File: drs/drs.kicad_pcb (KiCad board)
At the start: 2 copper layers, 68.5 x 53.5 mm, 26 parts, among them J1 CAN, J2 POWER, J3 BUTTON, J4 SERVO, U1 SN65HVD230, U2 TXU0202

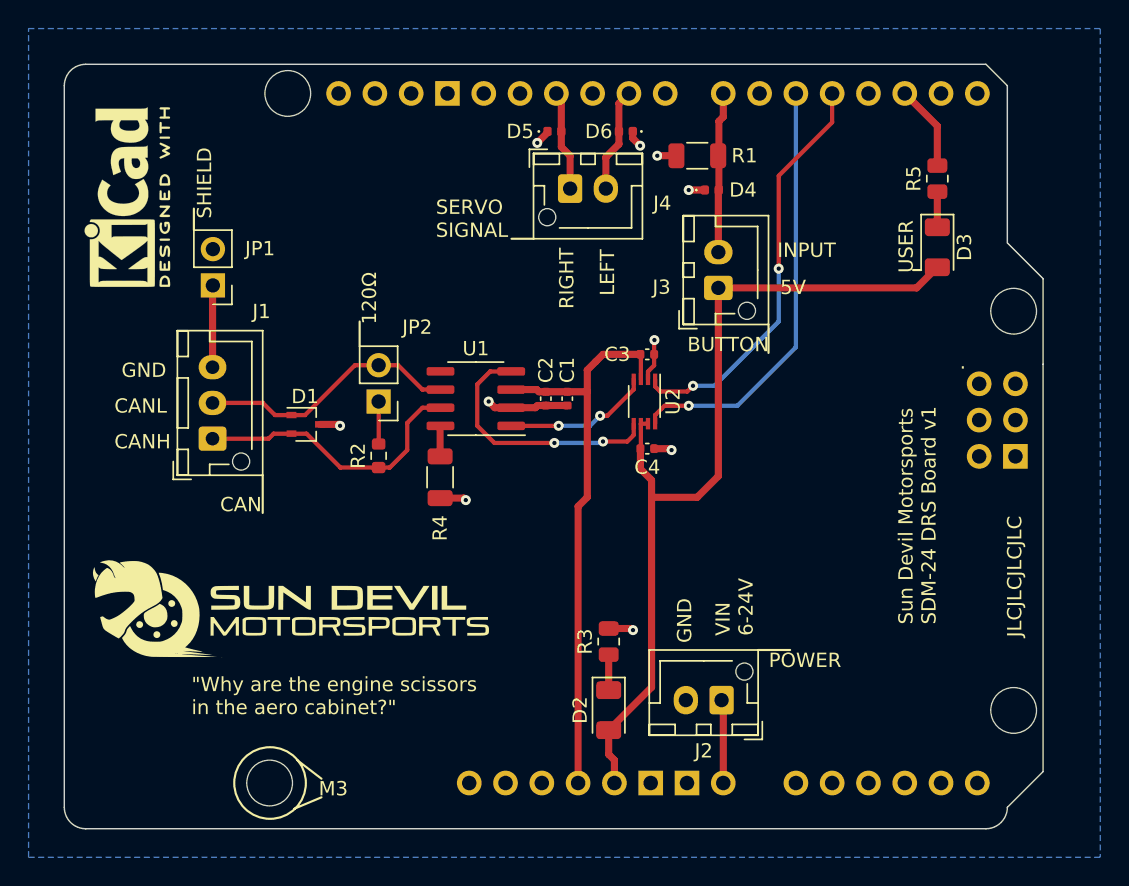
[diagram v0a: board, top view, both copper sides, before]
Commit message: fahb files
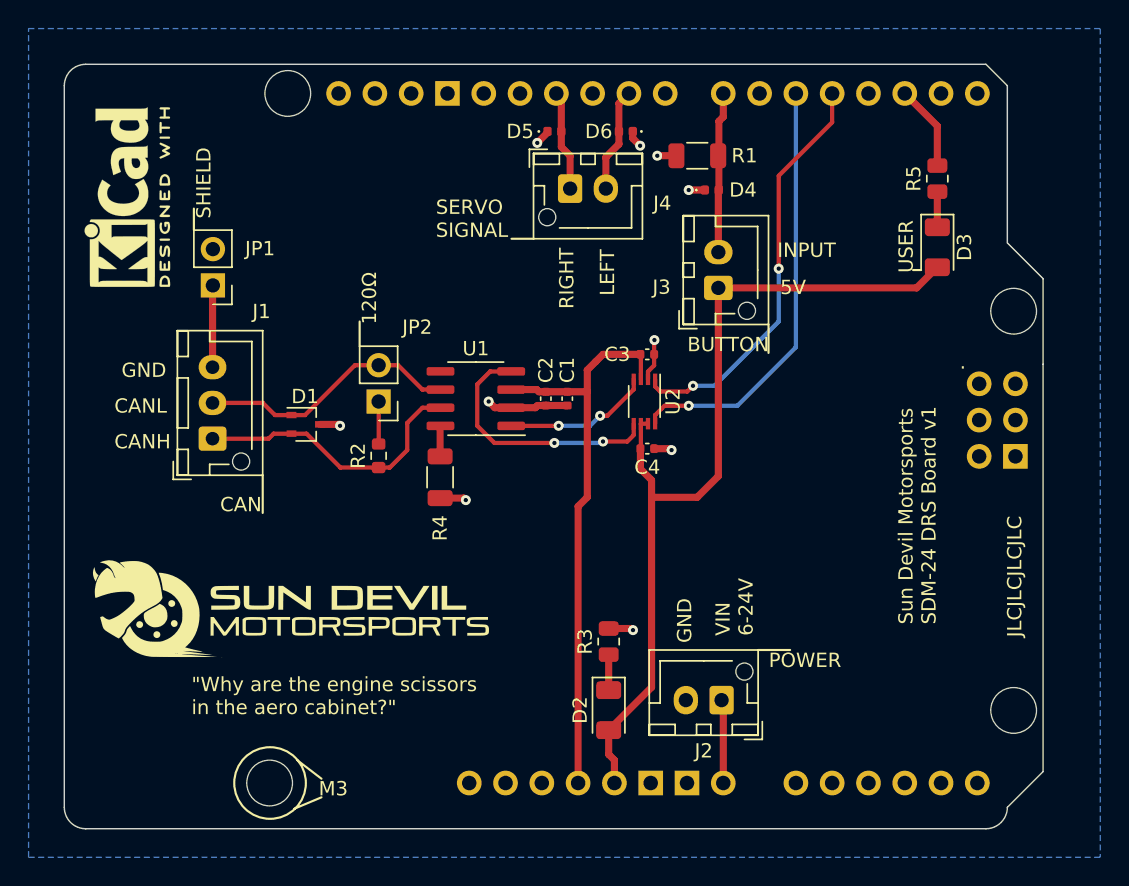
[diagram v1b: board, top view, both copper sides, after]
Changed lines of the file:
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@@
       (plot_on_all_layers_selection 0x0000000_00000000)
       (disableapertmacros false)
-      (usegerberextensions false)
-      (usegerberattributes true)
-      (usegerberadvancedattributes true)
-      (creategerberjobfile true)
+      (usegerberextensions true)
+      (usegerberattributes false)
+      (usegerberadvancedattributes false)
+      (creategerberjobfile false)
       (dashed_line_dash_ratio 12.000000)
       (dashed_line_gap_ratio 3.000000)
@@
       (psa4output false)
       (plotreference true)
-      (plotvalue true)
+      (plotvalue false)
       (plotinvisibletext false)
       (sketchpadsonfab false)
-      (subtractmaskfromsilk false)
+      (subtractmaskfromsilk true)
       (outputformat 1)
       (mirror false)
-      (drillshape 1)
+      (drillshape 0)
       (scaleselection 1)
-      (outputdirectory "")
+      (outputdirectory "fab/")
     )
   )
@@
       (stroke (width 0.1) (type solid)) (layer "F.Fab"))
     (pad "" np_thru_hole circle (at -1.6 2 90) (size 1.2 1.2) (drill 1.2) (layers "*.Cu" "*.Mask"))
-    (pad "1" thru_hole roundrect (at 0 0 90) (size 1.7 2) (drill 1) (layers "*.Cu" "*.Mask") (roundrect_rratio 0.147059)
+    (pad "1" thru_hole roundrect (at 0 0 90) (size 1.7 2) (drill 1) (layers "*.Cu" "*.Mask") (roundrect_rratio 0.1470588235)
       (net 40 "+5V") (pinfunction "Pin_1") (pintype "passive"))
     (pad "2" thru_hole oval (at 2.5 0 90) (size 1.7 2) (drill 1) (layers "*.Cu" "*.Mask")
@@
     (fp_line (start 1.6 0.8) (end -1.6 0.8)
       (stroke (width 0.1) (type solid)) (layer "F.Fab"))
-    (pad "1" smd roundrect (at -1.4625 0 180) (size 1.125 1.75) (layers "F.Cu" "F.Paste" "F.Mask") (roundrect_rratio 0.222222)
+    (pad "1" smd roundrect (at -1.4625 0 180) (size 1.125 1.75) (layers "F.Cu" "F.Paste" "F.Mask") (roundrect_rratio 0.2222222222)
       (net 17 "/BTN_INPUT") (pintype "passive"))
-    (pad "2" smd roundrect (at 1.4625 0 180) (size 1.125 1.75) (layers "F.Cu" "F.Paste" "F.Mask") (roundrect_rratio 0.222222)
+    (pad "2" smd roundrect (at 1.4625 0 180) (size 1.125 1.75) (layers "F.Cu" "F.Paste" "F.Mask") (roundrect_rratio 0.2222222222)
       (net 34 "GND") (pintype "passive"))
     (model "${KICAD6_3DMODEL_DIR}/Resistor_SMD.3dshapes/R_1206_3216Metric.wrl"
@@
     (fp_line (start 1 0.625) (end -1 0.625)
       (stroke (width 0.1) (type solid)) (layer "F.Fab"))
-    (pad "1" smd roundrect (at -0.9125 0 90) (size 1.025 1.4) (layers "F.Cu" "F.Paste" "F.Mask") (roundrect_rratio 0.243902)
+    (pad "1" smd roundrect (at -0.9125 0 90) (size 1.025 1.4) (layers "F.Cu" "F.Paste" "F.Mask") (roundrect_rratio 0.243902439)
       (net 44 "/PWR_LED") (pintype "passive"))
-    (pad "2" smd roundrect (at 0.9125 0 90) (size 1.025 1.4) (layers "F.Cu" "F.Paste" "F.Mask") (roundrect_rratio 0.243902)
+    (pad "2" smd roundrect (at 0.9125 0 90) (size 1.025 1.4) (layers "F.Cu" "F.Paste" "F.Mask") (roundrect_rratio 0.243902439)
       (net 34 "GND") (pintype "passive"))
     (model "${KICAD6_3DMODEL_DIR}/Resistor_SMD.3dshapes/R_0805_2012Metric.wrl"
@@
     (fp_line (start 1 0.625) (end -1 0.625)
       (stroke (width 0.1) (type solid)) (layer "F.Fab"))
-    (pad "1" smd roundrect (at -0.9125 0 90) (size 1.025 1.4) (layers "F.Cu" "F.Paste" "F.Mask") (roundrect_rratio 0.243902)
+    (pad "1" smd roundrect (at -0.9125 0 90) (size 1.025 1.4) (layers "F.Cu" "F.Paste" "F.Mask") (roundrect_rratio 0.243902439)
       (net 45 "/USR_LED_RSTR") (pintype "passive"))
-    (pad "2" smd roundrect (at 0.9125 0 90) (size 1.025 1.4) (layers "F.Cu" "F.Paste" "F.Mask") (roundrect_rratio 0.243902)
+    (pad "2" smd roundrect (at 0.9125 0 90) (size 1.025 1.4) (layers "F.Cu" "F.Paste" "F.Mask") (roundrect_rratio 0.243902439)
       (net 12 "/USR_LED") (pintype "passive"))
     (model "${KICAD6_3DMODEL_DIR}/Resistor_SMD.3dshapes/R_0805_2012Metric.wrl"
@@
     (fp_line (start 1.6 0.8) (end -1.6 0.8)
       (stroke (width 0.1) (type solid)) (layer "F.Fab"))
-    (pad "1" smd roundrect (at -1.4625 0 270) (size 1.125 1.75) (layers "F.Cu" "F.Paste" "F.Mask") (roundrect_rratio 0.222222)
+    (pad "1" smd roundrect (at -1.4625 0 270) (size 1.125 1.75) (layers "F.Cu" "F.Paste" "F.Mask") (roundrect_rratio 0.2222222222)
       (net 39 "/CAN_Rs") (pintype "passive"))
-    (pad "2" smd roundrect (at 1.4625 0 270) (size 1.125 1.75) (layers "F.Cu" "F.Paste" "F.Mask") (roundrect_rratio 0.222222)
+    (pad "2" smd roundrect (at 1.4625 0 270) (size 1.125 1.75) (layers "F.Cu" "F.Paste" "F.Mask") (roundrect_rratio 0.2222222222)
       (net 34 "GND") (pintype "passive"))
     (model "${KICAD6_3DMODEL_DIR}/Resistor_SMD.3dshapes/R_1206_3216Metric.wrl"
@@
       (stroke (width 0.1) (type solid)) (layer "F.Fab"))
     (pad "" np_thru_hole circle (at -1.6 2) (size 1.2 1.2) (drill 1.2) (layers "*.Cu" "*.Mask"))
-    (pad "1" thru_hole roundrect (at 0 0) (size 1.7 2) (drill 1) (layers "*.Cu" "*.Mask") (roundrect_rratio 0.147059)
+    (pad "1" thru_hole roundrect (at 0 0) (size 1.7 2) (drill 1) (layers "*.Cu" "*.Mask") (roundrect_rratio 0.1470588235)
       (net 21 "/SERVO_RIGHT") (pinfunction "Pin_1") (pintype "passive"))
     (pad "2" thru_hole oval (at 2.5 0) (size 1.7 2) (drill 1) (layers "*.Cu" "*.Mask")
@@
       (stroke (width 0.1) (type solid)) (layer "F.Fab"))
     (pad "" np_thru_hole circle (at -1.6 2 90) (size 1.2 1.2) (drill 1.2) (layers "*.Cu" "*.Mask"))
-    (pad "1" thru_hole roundrect (at 0 0 90) (size 1.7 1.95) (drill 0.95) (layers "*.Cu" "*.Mask") (roundrect_rratio 0.147059)
+    (pad "1" thru_hole roundrect (at 0 0 90) (size 1.7 1.95) (drill 0.95) (layers "*.Cu" "*.Mask") (roundrect_rratio 0.1470588235)
       (net 38 "/CANH") (pinfunction "Pin_1") (pintype "passive"))
     (pad "2" thru_hole oval (at 2.5 0 90) (size 1.7 1.95) (drill 0.95) (layers "*.Cu" "*.Mask")
@@
       (stroke (width 0.1) (type solid)) (layer "F.Fab"))
     (pad "" np_thru_hole circle (at -1.6 2 180) (size 1.2 1.2) (drill 1.2) (layers "*.Cu" "*.Mask"))
-    (pad "1" thru_hole roundrect (at 0 0 180) (size 1.7 2) (drill 1) (layers "*.Cu" "*.Mask") (roundrect_rratio 0.147059)
+    (pad "1" thru_hole roundrect (at 0 0 180) (size 1.7 2) (drill 1) (layers "*.Cu" "*.Mask") (roundrect_rratio 0.1470588235)
       (net 33 "VCC") (pinfunction "Pin_1") (pintype "passive"))
     (pad "2" thru_hole oval (at 2.5 0 180) (size 1.7 2) (drill 1) (layers "*.Cu" "*.Mask")
@@
     (effects (font (size 1 1) (thickness 0.15)) (justify left bottom))
   )
-  (gr_text "SHIELD" (at 124.9 80.3 90) (layer "F.SilkS" knockout)
+  (gr_text "SHIELD" (at 124.85 80.3 90) (layer "F.SilkS" knockout)
     (effects (font (size 1 1) (thickness 0.15)) (justify left bottom))
   )
